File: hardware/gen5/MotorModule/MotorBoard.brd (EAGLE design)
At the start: 160 x 100 mm, 49 parts, among them IC2 3.3V REG, J1 M20X2SHROUDED, M1O1 TEST_PT, M1O2 TEST_PT, M1O3 TEST_PT

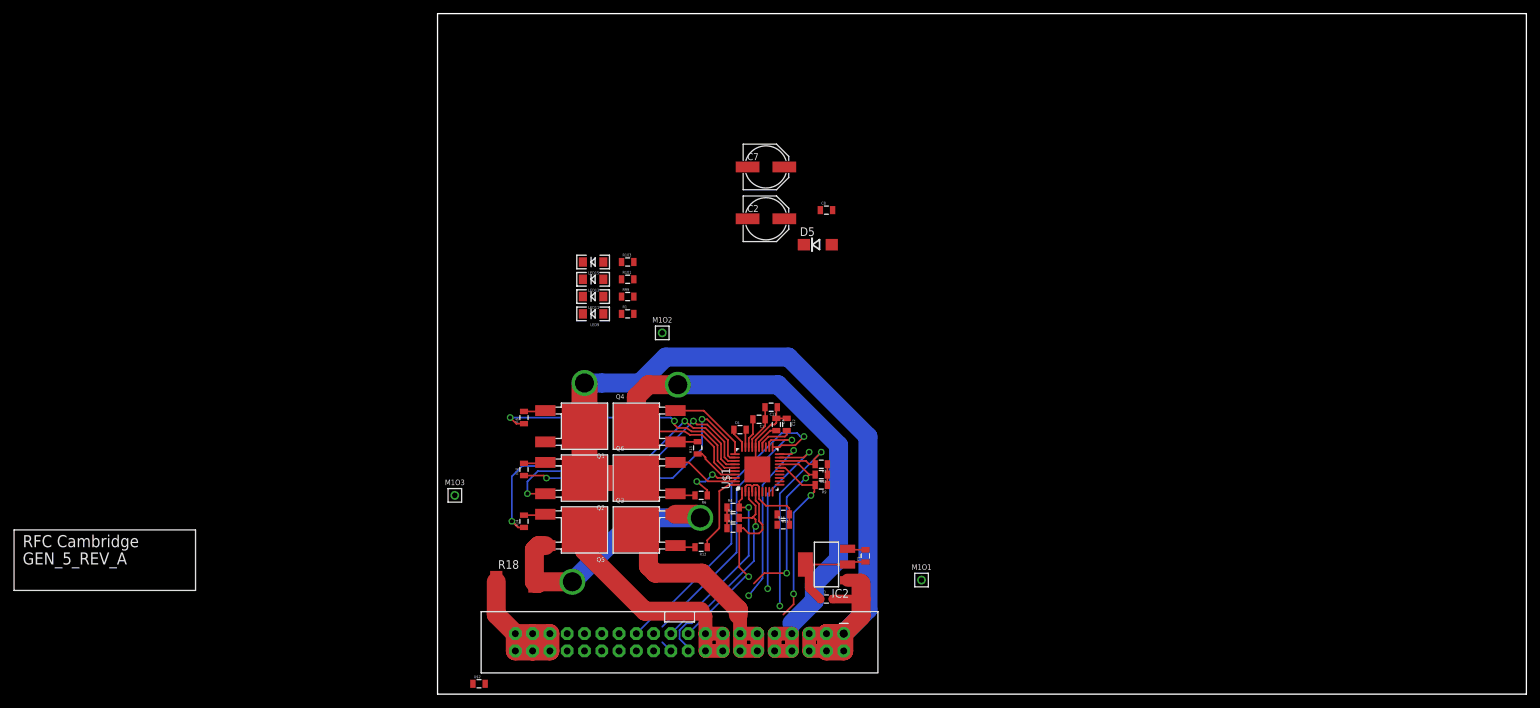
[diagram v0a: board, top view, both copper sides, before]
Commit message: Motor board finished - needs review
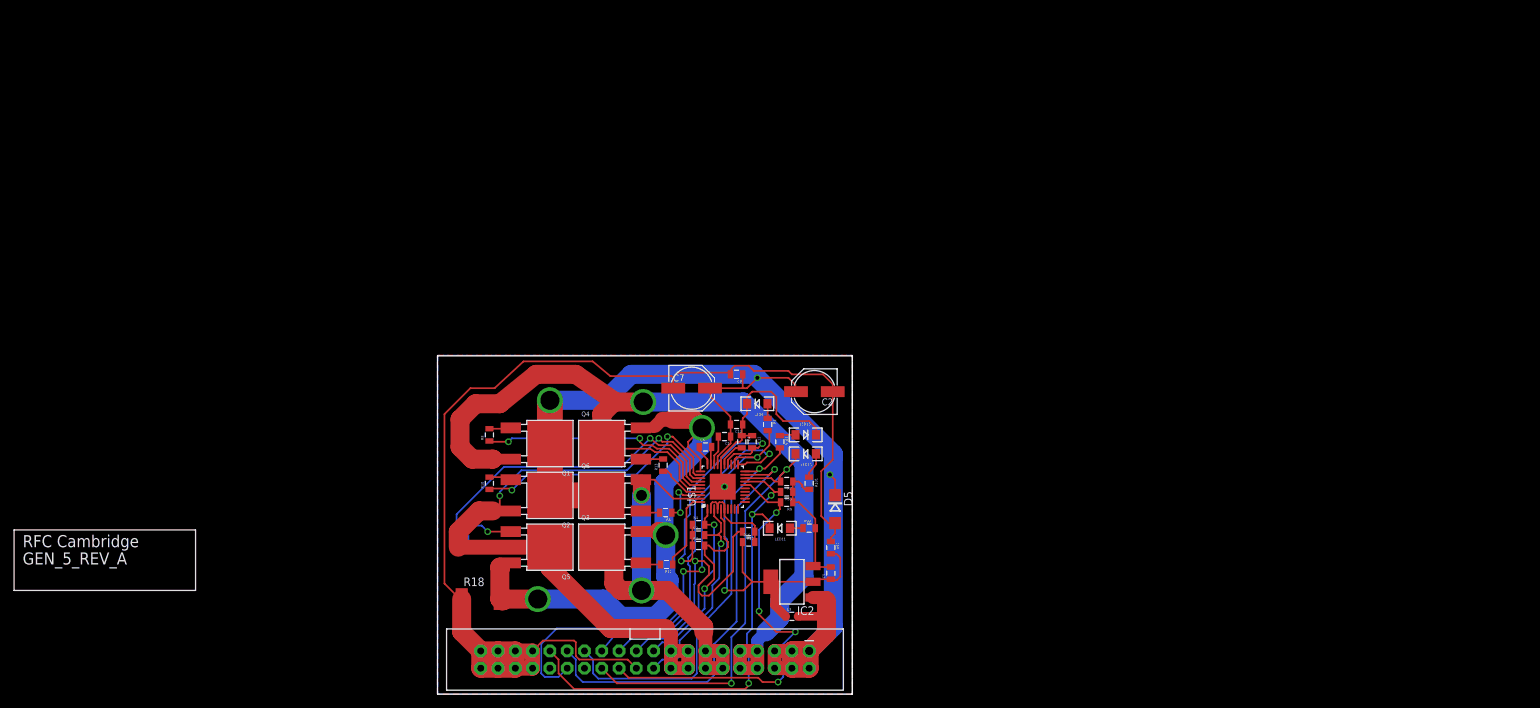
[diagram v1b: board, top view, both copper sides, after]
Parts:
- removed M1O1, M1O2, M1O3: TEST_PT, gen3:TESTING_PT
- moved U$2 55.4 mm to (57.8, 21.5), turned to 270 degrees
- moved LED11 43.7 mm to (50.3, 24.4)
- moved R99 43.2 mm to (54.6, 24.4)
- moved LED13 40.4 mm to (54.1, 35.3)
- moved LED15 40.3 mm to (54.1, 38.1), turned to 0 degrees
- moved R101 40.1 mm to (54.6, 31.0), turned to 270 degrees
- moved D5 38.9 mm to (58.4, 27.2), turned to 270 degrees
- moved R103 34.6 mm to (50.3, 37.1), turned to 270 degrees
- moved C7 34.3 mm to (37.3, 45.0)
- moved LED9 27.5 mm to (47.0, 42.7)
- moved C8 27.5 mm to (43.9, 47.0), turned to 180 degrees
- moved C2 26.4 mm to (55.4, 44.5), turned to 180 degrees
- moved R1 26.2 mm to (48.5, 39.6), turned to 270 degrees
- moved R14 8.77 mm to (4.06, 23.9), flipped to the bottom
- moved R6 5.79 mm to (33.5, 26.7)
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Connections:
- net 12VGND: now also J1.22, J1.33, J1.34
- net ENABLE: now also J1.30; no longer J1.22
- net M1O1: no longer M1O1.P$1
- net M1O2: no longer M1O2.P$1
- net M1O3: no longer M1O3.P$1
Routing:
- net 12VGND: track 26.6 -> 183.1 mm
- net 5V: track 8.36 -> 79.7 mm, vias 0 -> 3
- net GND: track 27.1 -> 83.1 mm, vias 0 -> 2
- net FAULTN: track 27.1 -> 73.0 mm, vias 2 -> 3
- net M1O2: track 97.7 -> 136.5 mm
- net PWM: track 27.3 -> 63.8 mm, vias 2 -> 1
- net HALLOUT: track 27.2 -> 63.1 mm, vias 2 -> 4
- net BRAKE: track 26.2 -> 60.6 mm, vias 2 -> 1
- net O1: track 51.4 -> 84.3 mm, vias 2 -> 3
- net LOCKN: track 32.8 -> 65.2 mm
- net 12V: track 142.2 -> 171.6 mm, vias 2 -> 4
- net ENABLE: track 41.9 -> 70.0 mm, vias 1 -> 3
- net M1O3: track 79.9 -> 101.6 mm
- net M1O1: track 45.6 -> 61.9 mm, vias 0 -> 2
- net 3.3V: track 5.72 -> 20.1 mm
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- added copper zone on layer 1, net 12VGND
- added copper zone on layer 16, net 12VGND
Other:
- board size 160 x 100 mm -> 60.9 x 49.7 mm
